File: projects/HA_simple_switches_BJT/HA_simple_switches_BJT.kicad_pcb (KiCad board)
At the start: 2 copper layers, 32.4 x 31.1 mm, 15 parts, among them J1 TerminalBlock_2pin, J2 TerminalBlock_3pin, J3 TerminalBlock_3pin, J4 TerminalBlock_3pin, J5 TerminalBlock_3pin, Q1 MMBT3904, Q2 MMBT3904, Q3 MMBT3904, T1 HA_simple_switches_BJT, T2 (C)UweHerting, T3 github.com/uherting/MyKiCADRep, T4 v0.101

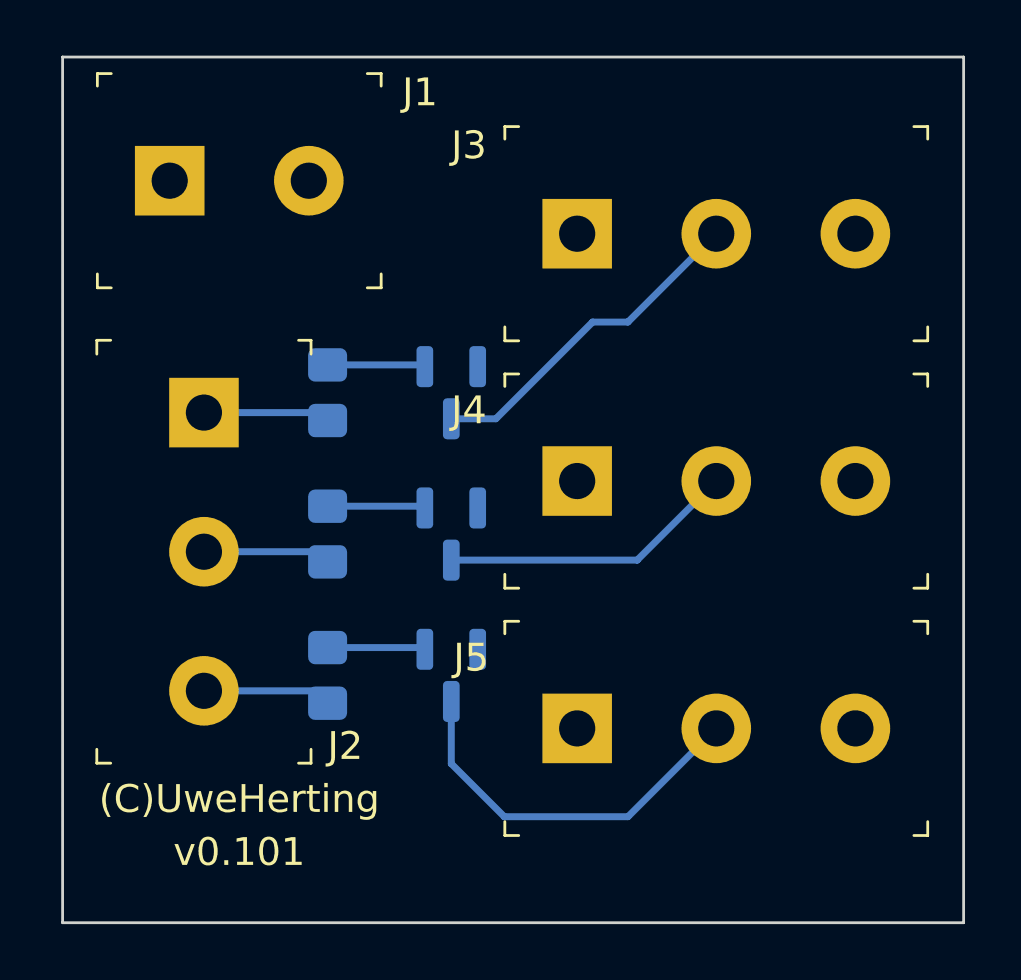
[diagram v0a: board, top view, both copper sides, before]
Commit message: snapshot
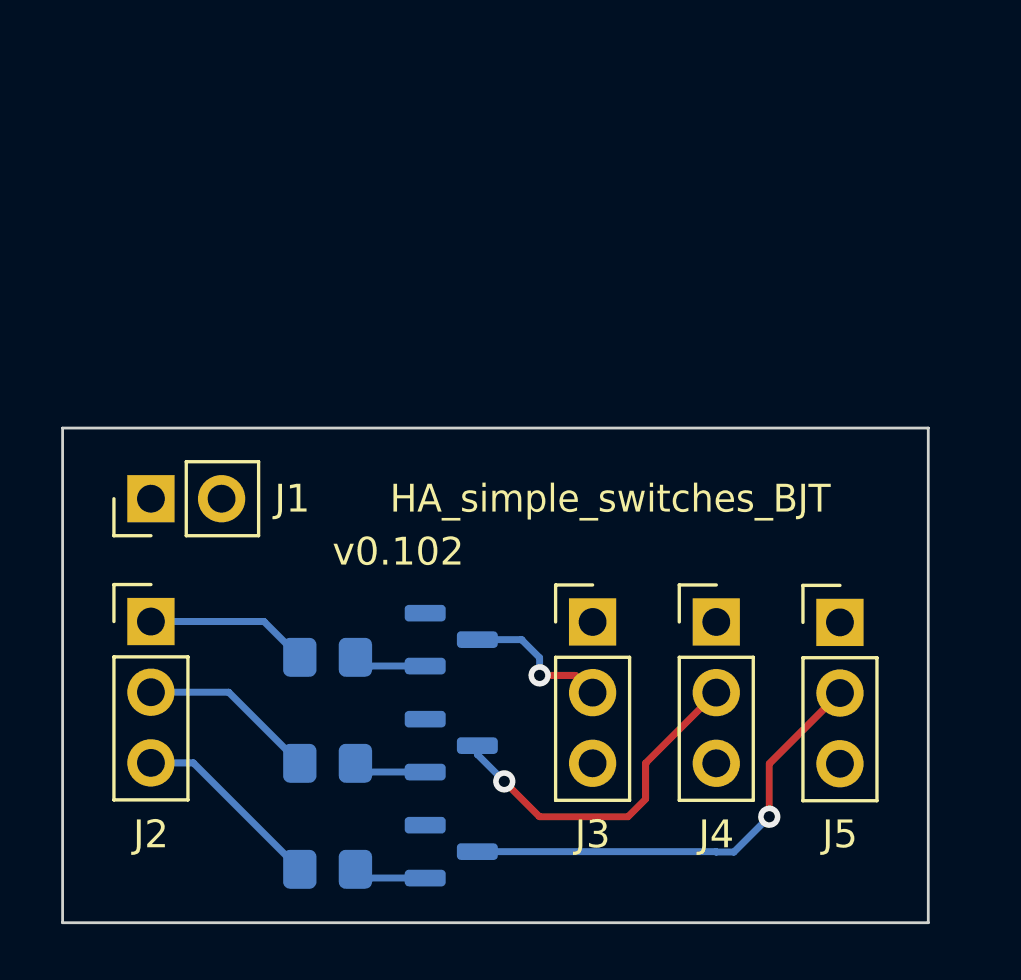
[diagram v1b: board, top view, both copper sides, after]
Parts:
- removed T2: (C)UweHerting, UH_HA:Copyright-Uwe_Herting
- removed T3: github.com/uherting/MyKiCADRep, UH_HA:GithubLink_UH
- J1: value TerminalBlock_2pin -> Conn_01x02_Pin; footprint UH_HA:Term_Block_1x2_P5mm -> Connector_PinHeader_2.54mm:PinHeader_1x02_P2.54mm_Vertical
- J2, J3, J4, J5: value TerminalBlock_3pin -> Conn_01x03_Pin; footprint UH_HA:Term_Block_1x3_P5mm -> Connector_PinHeader_2.54mm:PinHeader_1x03_P2.54mm_Vertical
- T1: moved to F.Cu
- T4: value v0.101 -> v0.102
- moved T1 14.8 mm to (156.8, 102.2), turned to 0 degrees
- moved J3 14.0 mm to (156.2, 106.0)
- moved T4 12.2 mm to (149.2, 104.1)
- moved J1 11.4 mm to (140.3, 101.6), turned to 90 degrees
- moved J5 10.2 mm to (165.1, 106.0)
- moved R1 9.51 mm to (146.7, 107.3), turned to 0 degrees
- moved Q1 8.88 mm to (151.1, 106.7), turned to 0 degrees
- moved R2 8.24 mm to (146.7, 111.1), turned to 0 degrees
- moved J2 7.75 mm to (140.3, 106.0), turned to 0 degrees
- moved Q2 7.60 mm to (151.1, 110.5), turned to 0 degrees
- moved J4 7.12 mm to (160.7, 106.0)
- moved R3 6.97 mm to (146.7, 114.9), turned to 0 degrees
- moved Q3 6.33 mm to (151.1, 114.3), turned to 0 degrees
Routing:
- net BJT_01: track 12.3 -> 5.30 mm, vias 0 -> 1
- net BJT_03: track 13.9 -> 16.5 mm, vias 0 -> 1
- net GPIO_3: track 4.63 -> 6.93 mm
- net GPIO_2: track 4.60 -> 6.41 mm
- net BJT_02: track 10.7 -> 12.4 mm, vias 0 -> 1
- net GPIO_1: track 4.56 -> 5.88 mm
- net Net-(Q3-B): track 3.52 -> 2.64 mm
- net Net-(Q2-B): track 3.52 -> 2.64 mm
- net Net-(Q1-B): track 3.52 -> 2.64 mm
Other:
- board size 32.4 x 31.1 mm -> 31.1 x 17.8 mm
